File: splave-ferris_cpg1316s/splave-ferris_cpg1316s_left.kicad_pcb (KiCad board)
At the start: 2 copper layers, 130.2 x 101.2 mm, 38 parts

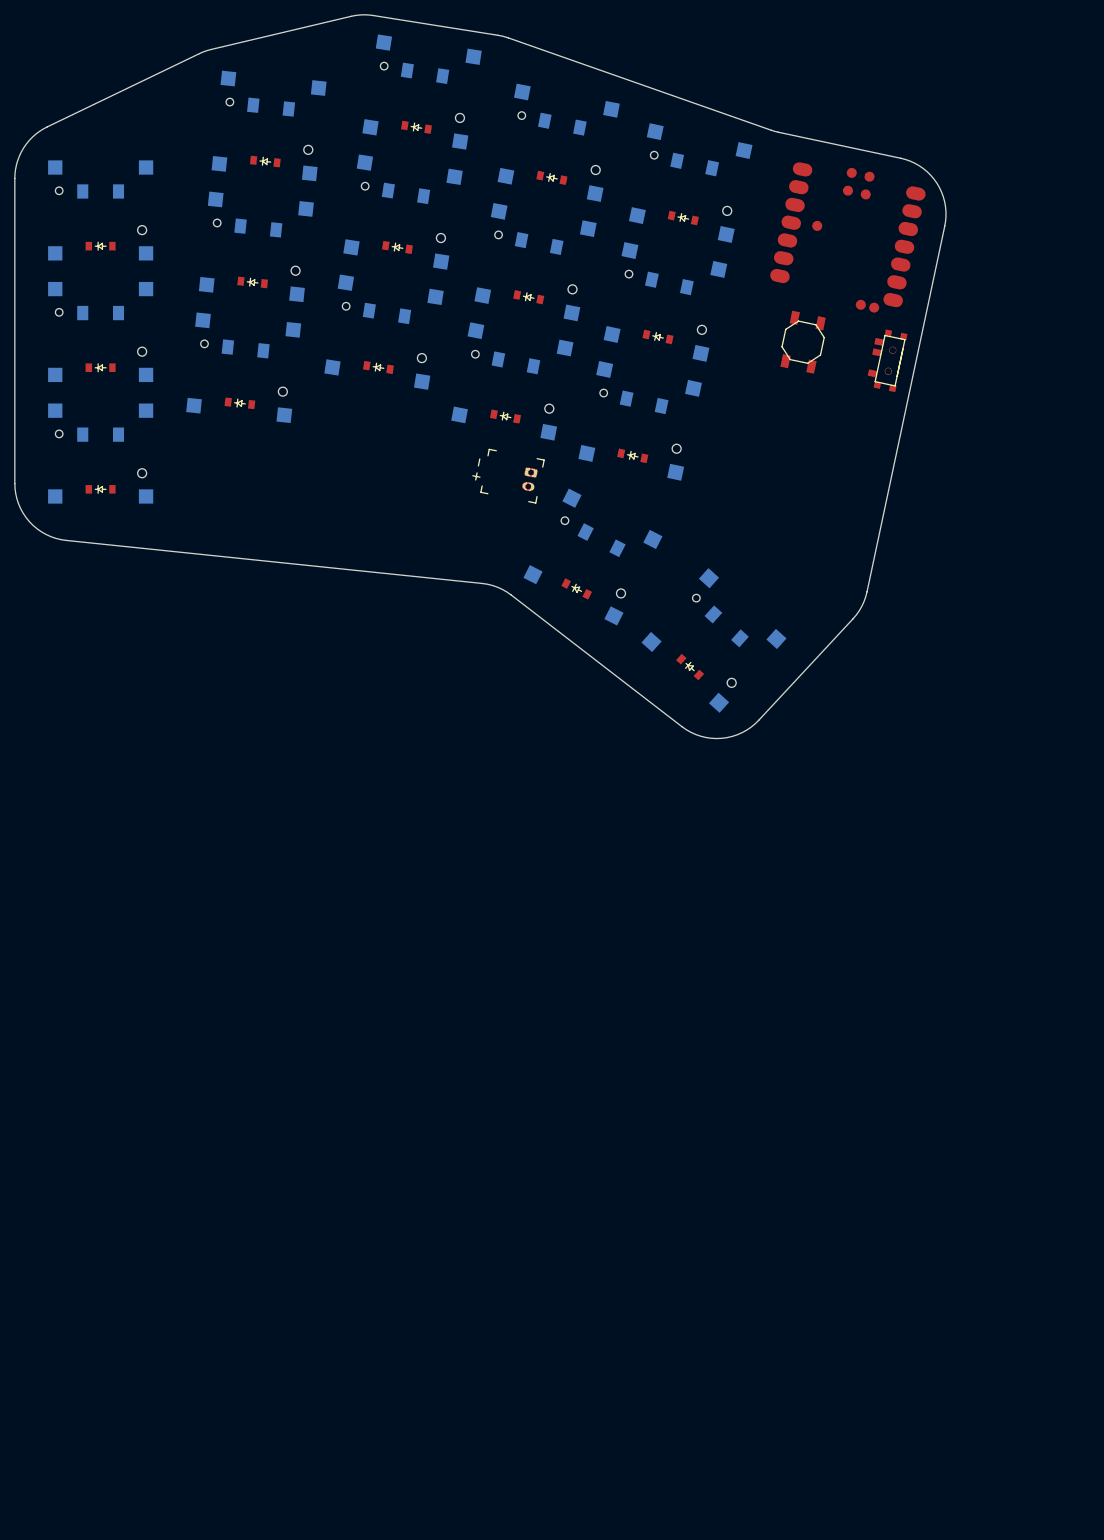
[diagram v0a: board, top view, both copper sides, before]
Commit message: Finalized choc_v1 design and created production files.
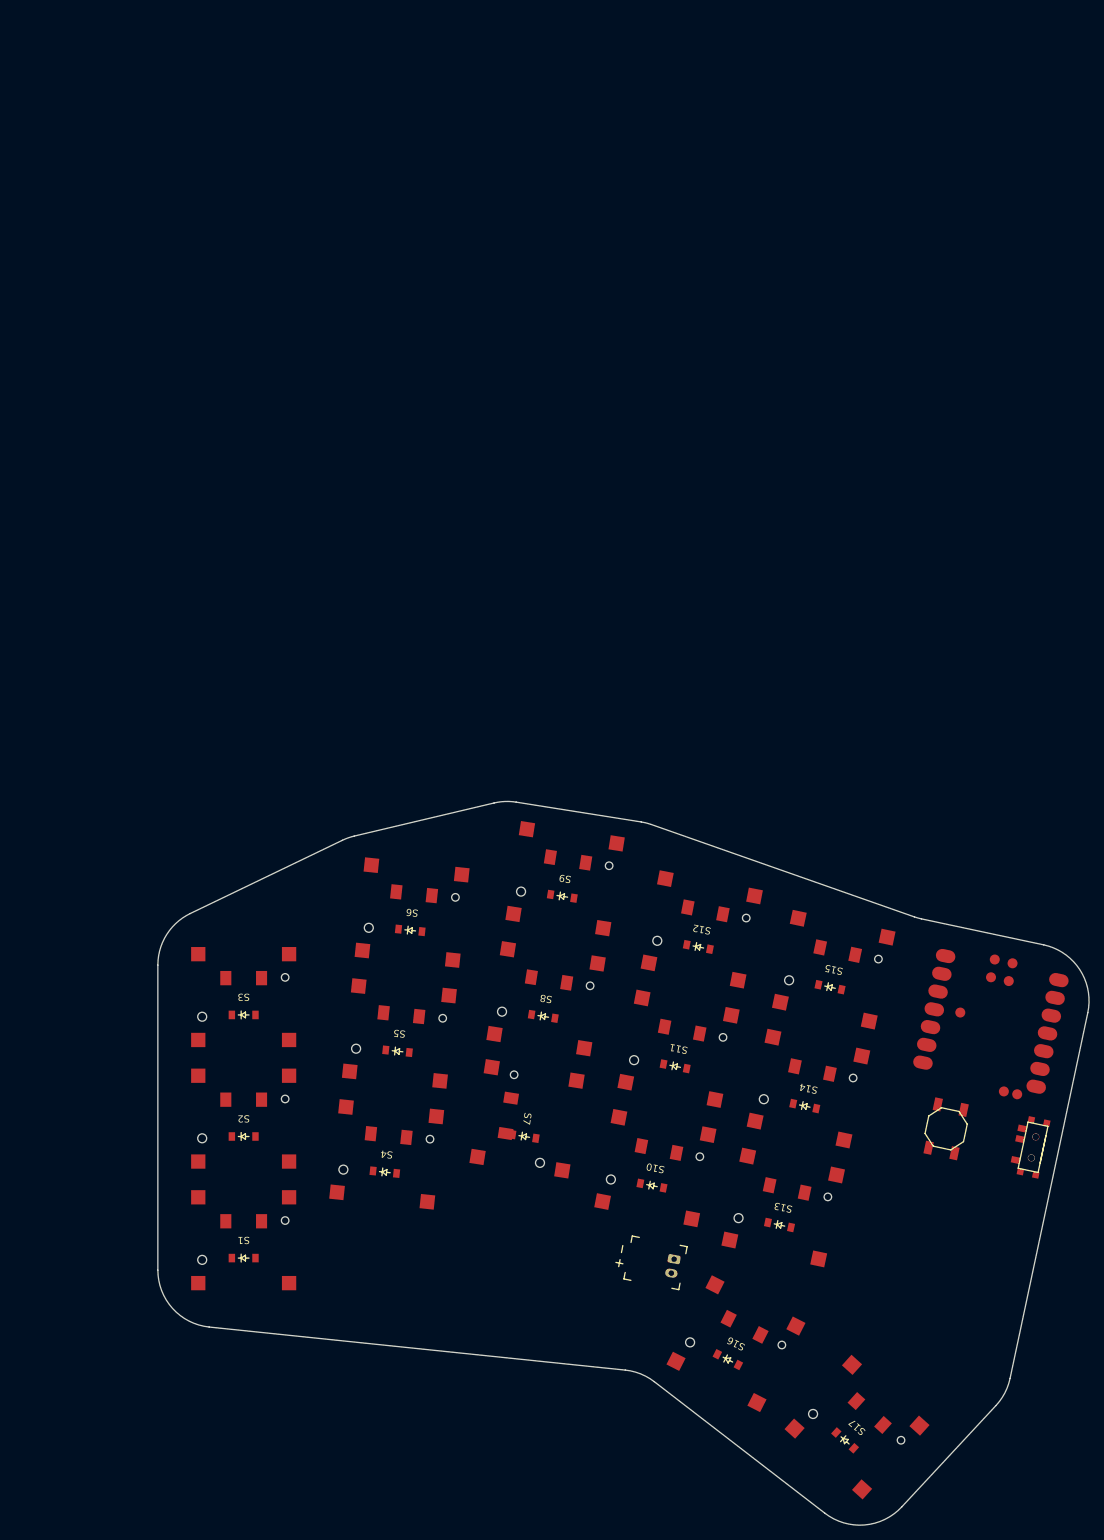
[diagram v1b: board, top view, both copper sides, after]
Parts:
- S1, S10, S11, S12, S13, S14, S15, S16, S17, S2, S3, S4, S5, S6, S7, S8, S9: moved to F.Cu
- moved JST1 111.8 mm to (180.0, 213.6)
- moved S11 111.8 mm to (180.8, 183.2), turned to 169 degrees
- moved S13 111.8 mm to (195.4, 205.4), turned to 168 degrees
- moved S16 111.8 mm to (188.8, 224.5), turned to 153 degrees
- moved S17 111.8 mm to (205.8, 236.1), turned to 138 degrees
- moved S5 111.8 mm to (141.8, 181.1), turned to 174 degrees
- moved S6 111.8 mm to (143.6, 164.2), turned to 174 degrees
- moved S7 111.8 mm to (159.6, 193.0), turned to -99 degrees
- moved T1 111.8 mm to (230.5, 197.0)
- moved B1 111.8 mm to (218.2, 194.4)
- moved MCU1 111.8 mm to (224.5, 179.4)
- moved S1 111.8 mm to (120.0, 210.0), turned to 180 degrees
- moved S10 111.8 mm to (177.6, 199.9), turned to 169 degrees
- moved S12 111.8 mm to (184.1, 166.5), turned to 169 degrees
- moved S14 111.8 mm to (199.0, 188.8), turned to 168 degrees
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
